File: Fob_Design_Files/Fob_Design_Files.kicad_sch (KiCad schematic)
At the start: 27 parts, among them IC2 TLV70030DDCT, U1 MAX16054AZT_T, U2 CC1101RGPR, U3 BU2032SM-JJ-GTR, U4 STM32C011F4Px, Y1 NX3225GA-26.000MHZ-EXS00A-CG0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

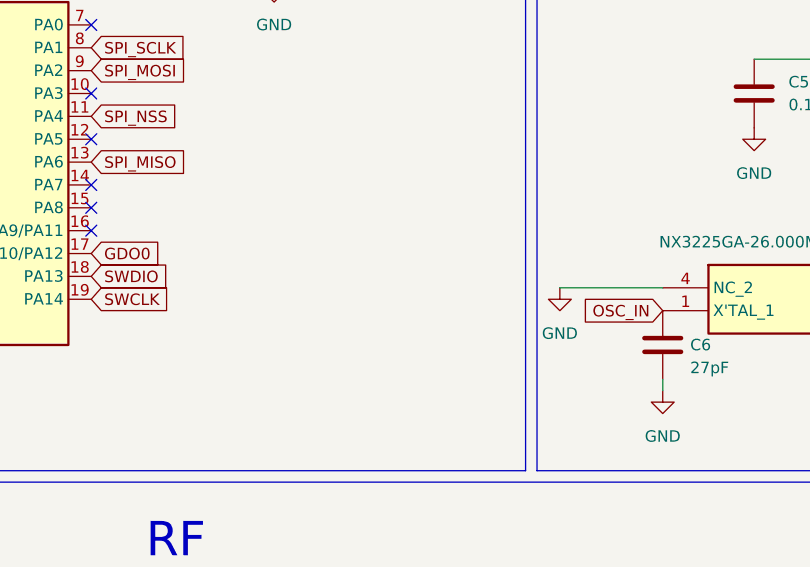
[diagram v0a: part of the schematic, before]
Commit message: Completed schematic
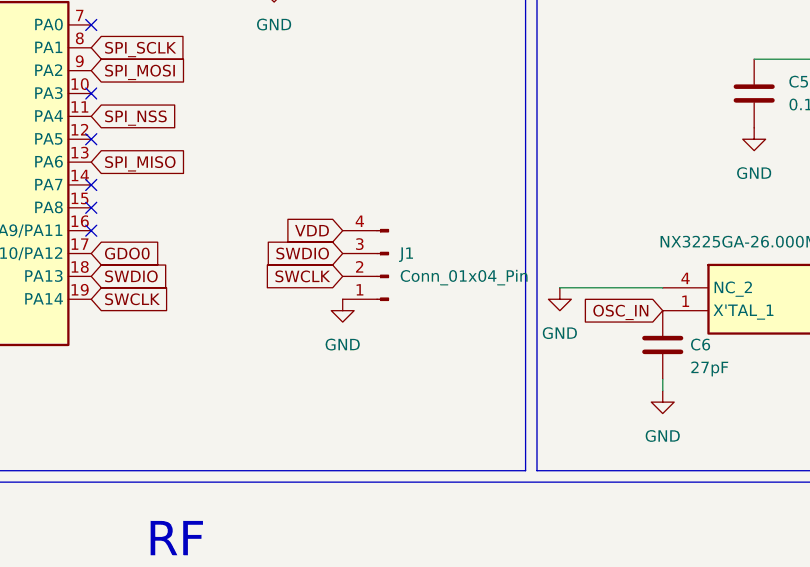
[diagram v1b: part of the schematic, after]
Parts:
- added J1: Conn_01x04_Pin, Connector_PinHeader_2.54mm:PinHeader_1x04_P2.54mm_Vertical, symbol Connector:Conn_01x04_Pin
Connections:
- net GND: now also J1.1 (Pin_1)
- net SWCLK: now also J1.2 (Pin_2)
- net SWDIO: now also J1.3 (Pin_3)
- net VDD: now also J1.4 (Pin_4)
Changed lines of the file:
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@@
 		)
 	)
+	(global_label "SWDIO"
+		(shape input)
+		(at 232.41 74.93 180)
+		(fields_autoplaced yes)
+		(effects
+			(font
+				(size 1.27 1.27)
+			)
+			(justify right)
+		)
+		(property "Intersheetrefs" "${INTERSHEET_REFS}"
+			(at 223.5586 74.93 0)
+			(effects
+				(font
+					(size 1.27 1.27)
+				)
+				(justify right)
+				(hide yes)
+			)
+		)
+	)
 	(global_label "RBIAS"
 		(shape input)
@@
 		)
 	)
+	(global_label "VDD"
+		(shape input)
+		(at 232.41 72.39 180)
+		(fields_autoplaced yes)
+		(effects
+			(font
+				(size 1.27 1.27)
+			)
+			(justify right)
+		)
+		(property "Intersheetrefs" "${INTERSHEET_REFS}"
+			(at 225.7962 72.39 0)
+			(effects
+				(font
+					(size 1.27 1.27)
+				)
+				(justify right)
+				(hide yes)
+			)
+		)
+	)
 	(global_label "SWDIO"
 		(shape input)
@@
 		)
 	)
+	(global_label "SWCLK"
+		(shape input)
+		(at 232.41 77.47 180)
+		(fields_autoplaced yes)
+		(effects
+			(font
+				(size 1.27 1.27)
+			)
+			(justify right)
+		)
+		(property "Intersheetrefs" "${INTERSHEET_REFS}"
+			(at 223.1958 77.47 0)
+			(effects
+				(font
+					(size 1.27 1.27)
+				)
+				(justify right)
+				(hide yes)
+			)
+		)
+	)
 	(symbol
 		(lib_id "SamacSys_Parts:BU2032SM-JJ-GTR")
@@
 	)
 	(symbol
+		(lib_id "Connector:Conn_01x04_Pin")
+		(at 237.49 77.47 180)
+		(unit 1)
+		(exclude_from_sim no)
+		(in_bom yes)
+		(on_board yes)
+		(dnp no)
+		(fields_autoplaced yes)
+		(property "Reference" "J1"
+			(at 238.76 74.9299 0)
+			(effects
+				(font
+					(size 1.27 1.27)
+				)
+				(justify right)
+			)
+		)
+		(property "Value" "Conn_01x04_Pin"
+			(at 238.76 77.4699 0)
+			(effects
+				(font
+					(size 1.27 1.27)
+				)
+				(justify right)
+			)
+		)
+		(property "Footprint" "Connector_PinHeader_2.54mm:PinHeader_1x04_P2.54mm_Vertical"
+			(at 237.49 77.47 0)
+			(effects
+				(font
+					(size 1.27 1.27)
+				)
+				(hide yes)
+			)
+		)
+		(property "Datasheet" "~"
+			(at 237.49 77.47 0)
+			(effects
+				(font
+					(size 1.27 1.27)
+				)
+				(hide yes)
+			)
+		)
+		(property "Description" "Generic connector, single row, 01x04, script generated"
+			(at 237.49 77.47 0)
+			(effects
+				(font
+					(size 1.27 1.27)
+				)
+				(hide yes)
+			)
+		)
+		(pin "1"
+		)
+		(pin "2"
+		)
+		(pin "4"
+		)
+		(pin "3"
+		)
+		(instances
+			(project ""
+				(path "/ad2bc408-bf54-4f88-a5fb-85c0e9c3efbd"
+					(reference "J1")
+					(unit 1)
+				)
+			)
+		)
+	)
+	(symbol
 		(lib_id "power:GND")
 		(at 224.79 44.45 0)
@@
 					(unit 1)
 				)
+			)
+		)
+	)
+	(symbol
+		(lib_id "power:GND")
+		(at 232.41 80.01 0)
+		(unit 1)
+		(exclude_from_sim no)
+		(in_bom yes)
+		(on_board yes)
+		(dnp no)
+		(fields_autoplaced yes)
+		(property "Reference" "#PWR027"
+			(at 232.41 86.36 0)
+			(effects
+				(font
+					(size 1.27 1.27)
+				)
+				(hide yes)
+			)
+		)
+		(property "Value" "GND"
+			(at 232.41 85.09 0)
+			(effects
+				(font
+					(size 1.27 1.27)
+				)
+			)
+		)
+		(property "Footprint" ""
+			(at 232.41 80.01 0)
+			(effects
+				(font
+					(size 1.27 1.27)
+				)
+				(hide yes)
+			)
+		)
+		(property "Datasheet" ""
+			(at 232.41 80.01 0)
+			(effects
+				(font
+					(size 1.27 1.27)
+				)
+				(hide yes)
+			)
+		)
+		(property "Description" "Power symbol creates a global label with name \"GND\" , ground"
+			(at 232.41 80.01 0)
+			(effects
+				(font
+					(size 1.27 1.27)
+				)
+				(hide yes)
+			)
+		)
+		(pin "1"
+		)
+		(instances
+			(project "Fob_Design_Files"
+				(path "/ad2bc408-bf54-4f88-a5fb-85c0e9c3efbd"
+					(reference "#PWR027")
+					(unit 1)
+				)
